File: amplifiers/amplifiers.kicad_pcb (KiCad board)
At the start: 2 copper layers, 4 parts, among them J1 Conn_01x03_Pin, J2 Conn_01x02_Pin, J3 Conn_01x03_Pin, U1 ADA4898-2

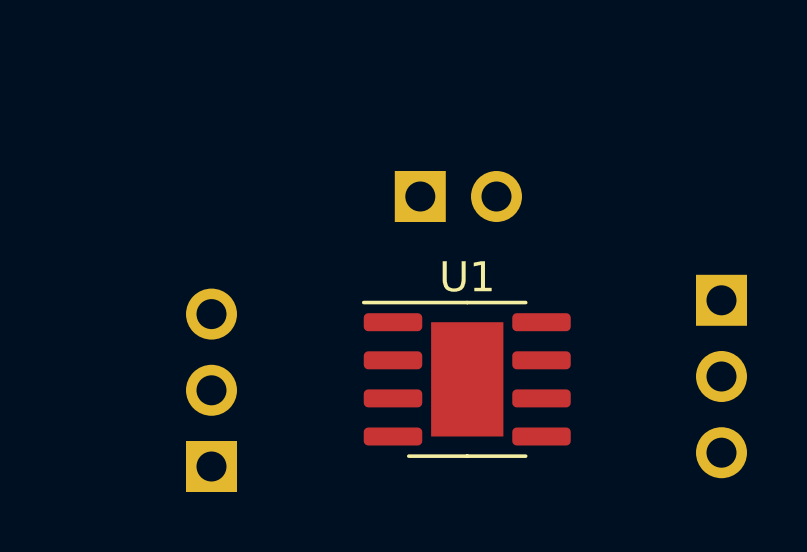
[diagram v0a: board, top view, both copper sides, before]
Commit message: Finishes version 0.1 of amplifier module board
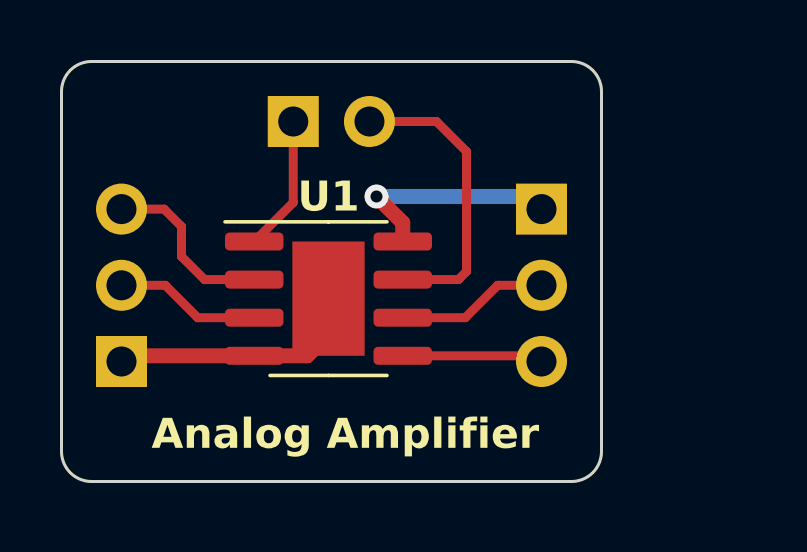
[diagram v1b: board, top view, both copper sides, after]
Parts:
- moved J3 6.73 mm to (151.0, 88.9)
- moved U1 5.35 mm to (143.9, 91.9)
- moved J2 4.92 mm to (142.7, 86.0)
- moved J1 4.61 mm to (137.0, 94.0)
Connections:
- U1 pad 5: Net-(J3-Pin_2) -> Net-(J3-Pin_3)
- U1 pad 6: Net-(J3-Pin_3) -> Net-(J3-Pin_2)
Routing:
- net Net-(J2-Pin_2): track 0.00 -> 9.89 mm
- net VEE: track 0.00 -> 8.55 mm
- net VDD: track 0.00 -> 7.54 mm, vias 0 -> 1
- net Net-(J1-Pin_3): track 0.00 -> 5.98 mm
- net Net-(J3-Pin_2): track 0.00 -> 5.07 mm
- net Net-(J1-Pin_2): track 0.00 -> 4.87 mm
- net Net-(J3-Pin_3): track 0.00 -> 4.70 mm
- net Net-(J2-Pin_1): track 0.00 -> 4.54 mm
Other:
- board outline added: 18 x 14 mm
- board text added: "+In1"
- board text added: "+In2"
- board text added: "+Vs"
- board text added: "-In1"
- board text added: "-In2"
- board text added: "-Vs"
- board text added: "Analog Amplifier"
- board text added: "Vo1"
- board text added: "Vo2"
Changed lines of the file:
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@@
   )
   (paper "A4")
+  (title_block
+    (title "Analog Amplifier Module Board PCB")
+    (date "2024-02-07")
+    (rev "0.1")
+    (company "Carlos Craveiro")
+    (comment 1 "Part of the Eibstein-Boltzmann Project")
+  )
   (layers
     (0 "F.Cu" signal)
@@
   (net 8 "Net-(J3-Pin_3)")
   (footprint "Package_SO:SOIC-8-1EP_3.9x4.9mm_P1.27mm_EP2.41x3.81mm" (layer "F.Cu")
-    (at 148.525 94.595)
+    (at 143.9 91.905)
     (descr "SOIC, 8 Pin (https://www.analog.com/media/en/technical-documentation/data-sheets/ada4898-1_4898-2.pdf#page=29), generated with kicad-footprint-generator ipc_gullwing_generator.py")
     (tags "SOIC SO")
@@
     (attr smd)
     (fp_text reference "U1" (at 0 -3.4) (layer "F.SilkS")
-        (effects (font (size 1 1) (thickness 0.15)))
+        (effects (font (size 1 1) (thickness 0.2) bold))
     )
     (fp_text value "ADA4898-2" (at 0 3.4) (layer "F.Fab")
@@
       (net 1 "VEE") (pinfunction "V-") (pintype "power_in"))
     (pad "5" smd roundrect (at 2.475 1.905) (size 1.95 0.6) (layers "F.Cu" "F.Paste" "F.Mask") (roundrect_rratio 0.25)
-      (net 7 "Net-(J3-Pin_2)") (pinfunction "+") (pintype "input"))
+      (net 8 "Net-(J3-Pin_3)") (pinfunction "+") (pintype "input"))
     (pad "6" smd roundrect (at 2.475 0.635) (size 1.95 0.6) (layers "F.Cu" "F.Paste" "F.Mask") (roundrect_rratio 0.25)
-      (net 8 "Net-(J3-Pin_3)") (pinfunction "-") (pintype "input"))
+      (net 7 "Net-(J3-Pin_2)") (pinfunction "-") (pintype "input"))
     (pad "7" smd roundrect (at 2.475 -0.635) (size 1.95 0.6) (layers "F.Cu" "F.Paste" "F.Mask") (roundrect_rratio 0.25)
       (net 5 "Net-(J2-Pin_2)") (pintype "output"))
@@
       (rotate (xyz 0 0 0))
     )
+    (model "/home/coveiro/Documents/Zedney/einstein-boltzmann/tension-multiplier/R_8_ADI.step"
+      (offset (xyz 0 0 0))
+      (scale (xyz 1 1 1))
+      (rotate (xyz 0 0 0))
+    )
   )
   (footprint "Connector_PinHeader_2.54mm:PinHeader_1x03_P2.54mm_Vertical" (layer "B.Cu")
-    (at 157 91.96 180)
+    (at 151 88.92 180)
     (descr "Through hole straight pin header, 1x03, 2.54mm pitch, single row")
     (tags "Through hole pin header THT 1x03 2.54mm single row")
@@
     (property "ki_keywords" "connector")
     (attr through_hole)
-    (fp_text reference "J3" (at 0 2.33) (layer "B.SilkS")
-        (effects (font (size 1 1) (thickness 0.15)) (justify mirror))
+    (fp_text reference "J3" (at 0 -7.58) (layer "B.SilkS")
+        (effects (font (size 1 1) (thickness 0.2) bold) (justify mirror))
     )
     (fp_text value "Conn_01x03_Pin" (at 0 -7.41) (layer "B.Fab")
@@
   )
   (footprint "Connector_PinHeader_2.54mm:PinHeader_1x03_P2.54mm_Vertical" (layer "B.Cu")
-    (at 140 97.5)
+    (at 137 94)
     (descr "Through hole straight pin header, 1x03, 2.54mm pitch, single row")
     (tags "Through hole pin header THT 1x03 2.54mm single row")
@@
     (attr through_hole)
     (fp_text reference "J1" (at 0 2.33) (layer "B.SilkS")
-        (effects (font (size 1 1) (thickness 0.15)) (justify mirror))
+        (effects (font (size 1 1) (thickness 0.2) bold) (justify mirror))
     )
     (fp_text value "Conn_01x03_Pin" (at 0 -7.41) (layer "B.Fab")
@@
   )
   (footprint "Connector_PinHeader_2.54mm:PinHeader_1x02_P2.54mm_Vertical" (layer "B.Cu")
-    (at 146.96 88.5 -90)
+    (at 142.725 86 -90)
     (descr "Through hole straight pin header, 1x02, 2.54mm pitch, single row")
     (tags "Through hole pin header THT 1x02 2.54mm single row")
@@
     (property "ki_keywords" "connector")
     (attr through_hole)
-    (fp_text reference "J2" (at 0 2.33 90) (layer "B.SilkS")
-        (effects (font (size 1 1) (thickness 0.15)) (justify mirror))
+    (fp_text reference "J2" (at 2.5 -1.275) (layer "B.SilkS")
+        (effects (font (size 1 1) (thickness 0.2) bold) (justify mirror))
     )
     (fp_text value "Conn_01x02_Pin" (at 0 -4.87 90) (layer "B.Fab")
@@
     )
   )
+  (gr_arc (start 152 84) (mid 152.707107 84.292893) (end 153 85)
+    (stroke (width 0.1) (type default)) (layer "Edge.Cuts"))
+  (gr_arc (start 136 98) (mid 135.292893 97.707107) (end 135 97)
+    (stroke (width 0.1) (type default)) (layer "Edge.Cuts"))
+  (gr_arc (start 135 85) (mid 135.292893 84.292893) (end 136 84)
+    (stroke (width 0.1) (type default)) (layer "Edge.Cuts"))
+  (gr_line (start 136 98) (end 152 98)
+    (stroke (width 0.1) (type default)) (layer "Edge.Cuts"))
+  (gr_arc (start 153 97) (mid 152.707107 97.707107) (end 152 98)
+    (stroke (width 0.1) (type default)) (layer "Edge.Cuts"))
+  (gr_line (start 153 85) (end 153 97)
+    (stroke (width 0.1) (type default)) (layer "Edge.Cuts"))
+  (gr_line (start 136 84) (end 152 84)
+    (stroke (width 0.1) (type default)) (layer "Edge.Cuts"))
+  (gr_line (start 135 85) (end 135 97)
+    (stroke (width 0.1) (type default)) (layer "Edge.Cuts"))
+  (gr_text "+In1" (at 142.5 92) (layer "B.SilkS")
+    (effects (font (size 1 1) (thickness 0.2) bold) (justify left bottom mirror))
+  )
+  (gr_text "Vo1" (at 141 86.5) (layer "B.SilkS")
+    (effects (font (size 1 1) (thickness 0.2) bold) (justify left bottom mirror))
+  )
+  (gr_text "+Vs" (at 149.5 89.5) (layer "B.SilkS")
+    (effects (font (size 1 1) (thickness 0.2) bold) (justify left bottom mirror))
+  )
+  (gr_text "-In2" (at 149.5 92) (layer "B.SilkS")
+    (effects (font (size 1 1) (thickness 0.2) bold) (justify left bottom mirror))
+  )
+  (gr_text "-Vs" (at 142 94.5) (layer "B.SilkS")
+    (effects (font (size 1 1) (thickness 0.2) bold) (justify left bottom mirror))
+  )
+  (gr_text "+In2" (at 149.5 94.5) (layer "B.SilkS")
+    (effects (font (size 1 1) (thickness 0.2) bold) (justify left bottom mirror))
+  )
+  (gr_text "Vo2" (at 150 86.5) (layer "B.SilkS")
+    (effects (font (size 1 1) (thickness 0.2) bold) (justify left bottom mirror))
+  )
+  (gr_text "-In1" (at 142.5 89.5) (layer "B.SilkS")
+    (effects (font (size 1 1) (thickness 0.2) bold) (justify left bottom mirror))
+  )
+  (gr_text "Analog Amplifier" (at 138 97) (layer "F.SilkS")
+    (effects (font (size 1 1) (thickness 0.2) bold) (justify left bottom))
+  )
+  (segment (start 141.425 93.81) (end 137.19 93.81) (width 0.5) (layer "F.Cu") (net 1))
+  (segment (start 143.9 91.905) (end 144 92.005) (width 0.5) (layer "F.Cu") (net 1))
+  (segment (start 144 93) (end 143.19 93.81) (width 0.5) (layer "F.Cu") (net 1))
+  (segment (start 144 92.005) (end 144 93) (width 0.5) (layer "F.Cu") (net 1))
+  (segment (start 143.19 93.81) (end 141.425 93.81) (width 0.5) (layer "F.Cu") (net 1))
+  (segment (start 137.19 93.81) (end 137 94) (width 0.5) (layer "F.Cu") (net 1))
+  (segment (start 138.46 91.46) (end 137 91.46) (width 0.3) (layer "F.Cu") (net 2))
+  (segment (start 139.54 92.54) (end 138.46 91.46) (width 0.3) (layer "F.Cu") (net 2))
+  (segment (start 141.425 92.54) (end 139.54 92.54) (width 0.3) (layer "F.Cu") (net 2))
+  (segment (start 138.42 88.92) (end 139 89.5) (width 0.3) (layer "F.Cu") (net 3))
+  (segment (start 139.77 91.27) (end 141.425 91.27) (width 0.3) (layer "F.Cu") (net 3))
+  (segment (start 139 90.5) (end 139.77 91.27) (width 0.3) (layer "F.Cu") (net 3))
+  (segment (start 139 89.5) (end 139 90.5) (width 0.3) (layer "F.Cu") (net 3))
+  (segment (start 137 88.92) (end 138.42 88.92) (width 0.3) (layer "F.Cu") (net 3))
+  (segment (start 142.725 86) (end 142.725 88.7) (width 0.3) (layer "F.Cu") (net 4))
+  (segment (start 142.725 88.7) (end 141.425 90) (width 0.3) (layer "F.Cu") (net 4))
+  (segment (start 148.23 91.27) (end 148.5 91) (width 0.3) (layer "F.Cu") (net 5))
+  (segment (start 148.5 87) (end 147.5 86) (width 0.3) (layer "F.Cu") (net 5))
+  (segment (start 146.375 91.27) (end 148.23 91.27) (width 0.3) (layer "F.Cu") (net 5))
+  (segment (start 148.5 91) (end 148.5 87) (width 0.3) (layer "F.Cu") (net 5))
+  (segment (start 147.5 86) (end 145.265 86) (width 0.3) (layer "F.Cu") (net 5))
+  (segment (start 146.375 89.375) (end 146.375 90) (width 0.5) (layer "F.Cu") (net 6))
+  (segment (start 145.5 88.5) (end 146.375 89.375) (width 0.5) (layer "F.Cu") (net 6))
+  (via (at 145.5 88.5) (size 0.8) (drill 0.4) (layers "F.Cu" "B.Cu") (net 6))
+  (segment (start 145.5 88.5) (end 150.58 88.5) (width 0.5) (layer "B.Cu") (net 6))
+  (segment (start 150.58 88.5) (end 151 88.92) (width 0.5) (layer "B.Cu") (net 6))
+  (segment (start 149.54 91.46) (end 151 91.46) (width 0.3) (layer "F.Cu") (net 7))
+  (segment (start 146.375 92.54) (end 148.46 92.54) (width 0.3) (layer "F.Cu") (net 7))
+  (segment (start 148.46 92.54) (end 149.54 91.46) (width 0.3) (layer "F.Cu") (net 7))
+  (segment (start 150.81 93.81) (end 151 94) (width 0.3) (layer "F.Cu") (net 8))
+  (segment (start 146.375 93.81) (end 150.81 93.81) (width 0.3) (layer "F.Cu") (net 8))
 )
